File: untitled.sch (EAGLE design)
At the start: 35 parts, among them J1 61300311121, Q1 FQPF10N60C, Q2 2N3906, T1 S8050, T2 s8050, T3 s8050

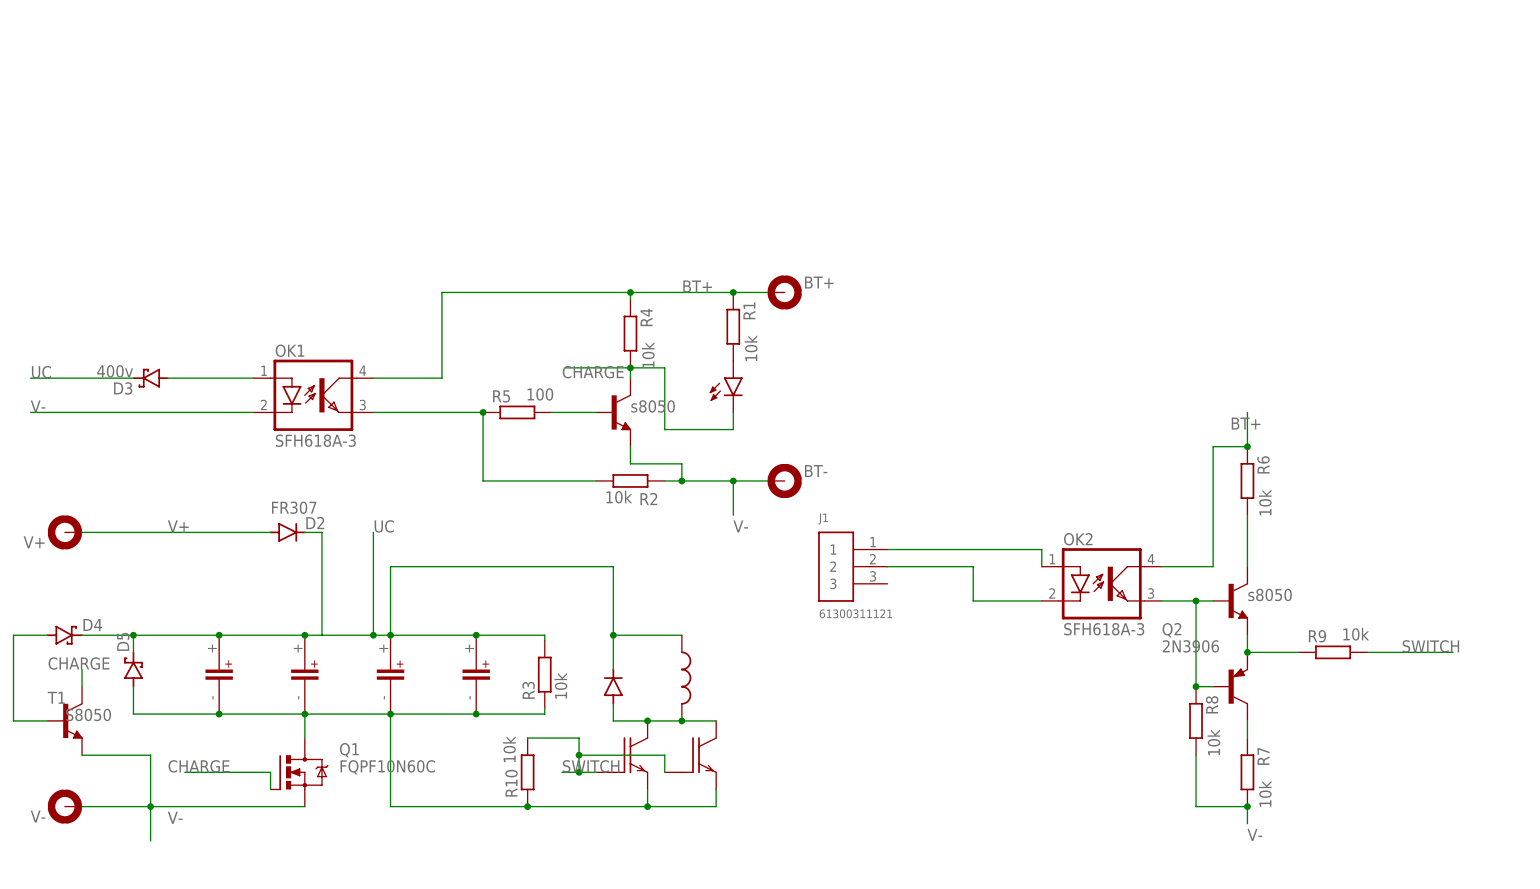
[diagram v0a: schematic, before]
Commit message: add
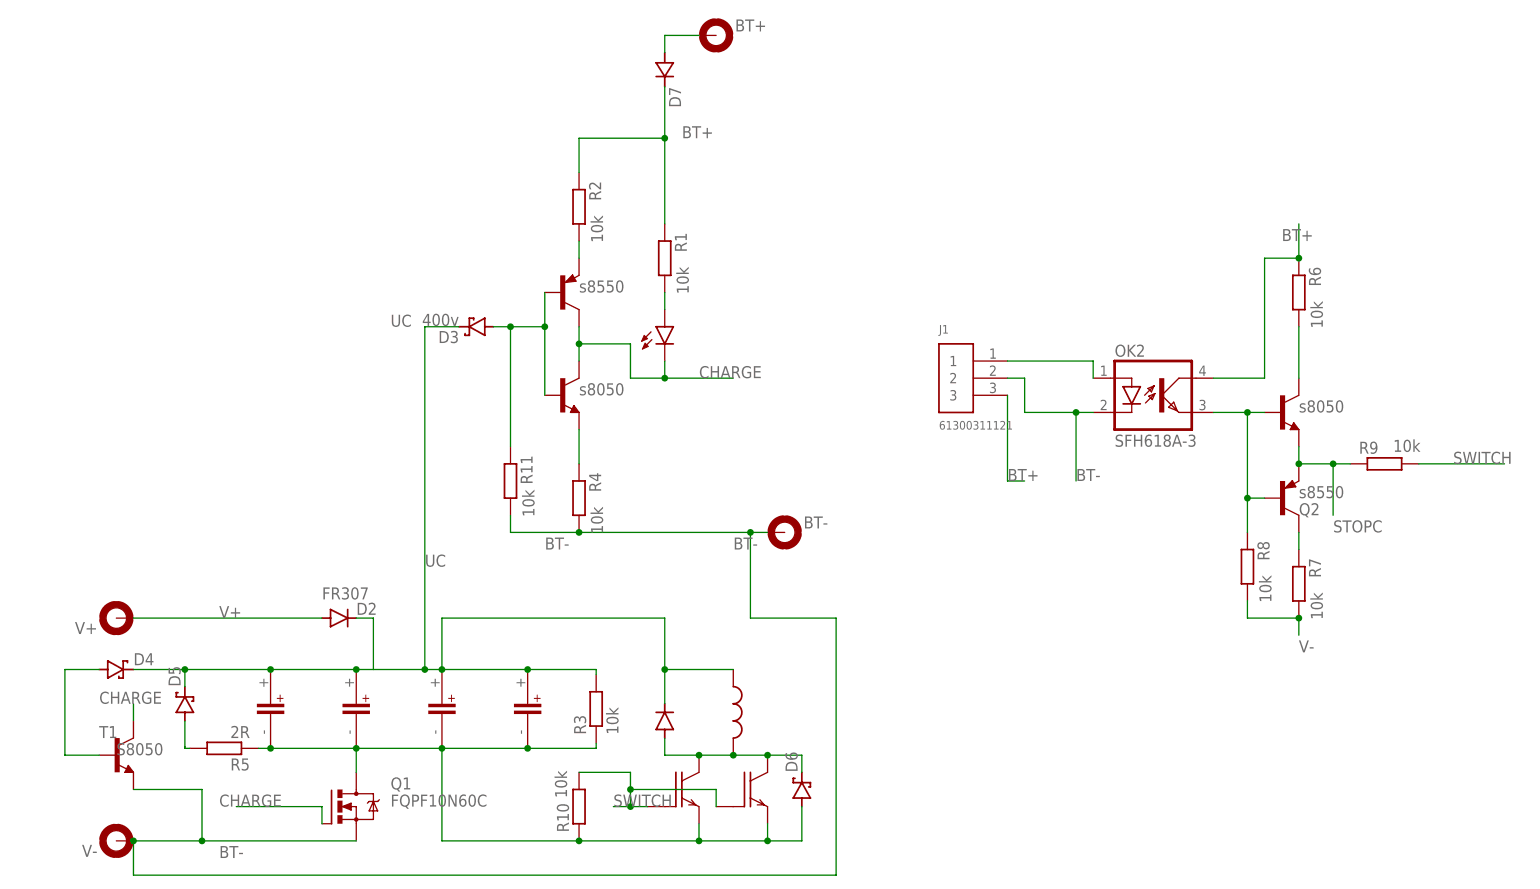
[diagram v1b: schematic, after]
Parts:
- removed OK1: SFH618A-3, optocoupler:SFH618A-3
- added D6: (no value), zetex:DS_E2L
- added D7: (no value), zetex:D_E2L
- added Q3: s8550, transistor-pnp:2N3906
- added R11: 10k, rcl:R-EU_0207/2V
- Q2: value 2N3906 -> s8550
- R5: value 100 -> 2R
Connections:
- net N$8 renamed STOPC
- removed net N$5: OK1.EMIT, R2.1, R5.1
- removed net V2-: J1.2, OK2.C
- new net BT-: BT-.MOUNT, J1.2, OK2.C, Q1.S, R11.2, R4.2, T1.E, V-.MOUNT
- new net N$7: D3.A, Q3.B, R11.1, T2.B
- new net N$8: R4.1, T2.E
- new net N$9: Q3.E, R2.2
- net BT+: now also D7.C, J1.3, R2.1; no longer BT+.MOUNT, OK1.COL, R4.1
- net CHARGE: now also Q3.C; no longer R4.2
- net N$10: now also D6.A, R5.1; no longer D5.A
- net N$2: now also BT+.MOUNT, D7.A; no longer D3.A, OK1.A
- net N$3: now also D5.A; no longer T2.B
- net N$4: now also D6.K
- net V-: no longer BT-.MOUNT, OK1.C, Q1.S, R2.2, T1.E, T2.E, V-.MOUNT
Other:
- moved on the sheet: BT+, BT-, D2, D3, D4, D5, J1, OK2, Q1, Q2, R1, R10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
